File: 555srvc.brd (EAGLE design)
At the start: 34 x 27.9 mm, 11 parts, among them IC2 NE555P

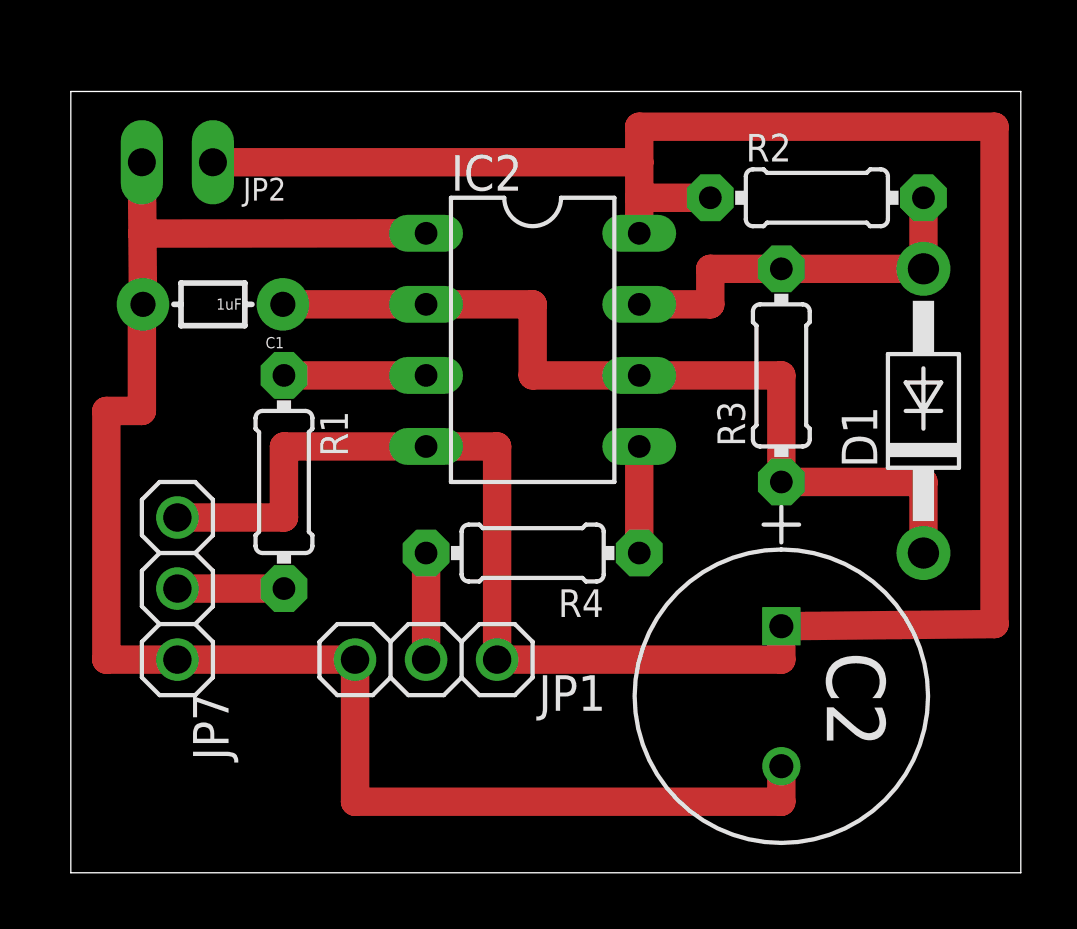
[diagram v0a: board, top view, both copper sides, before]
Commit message: smd is go
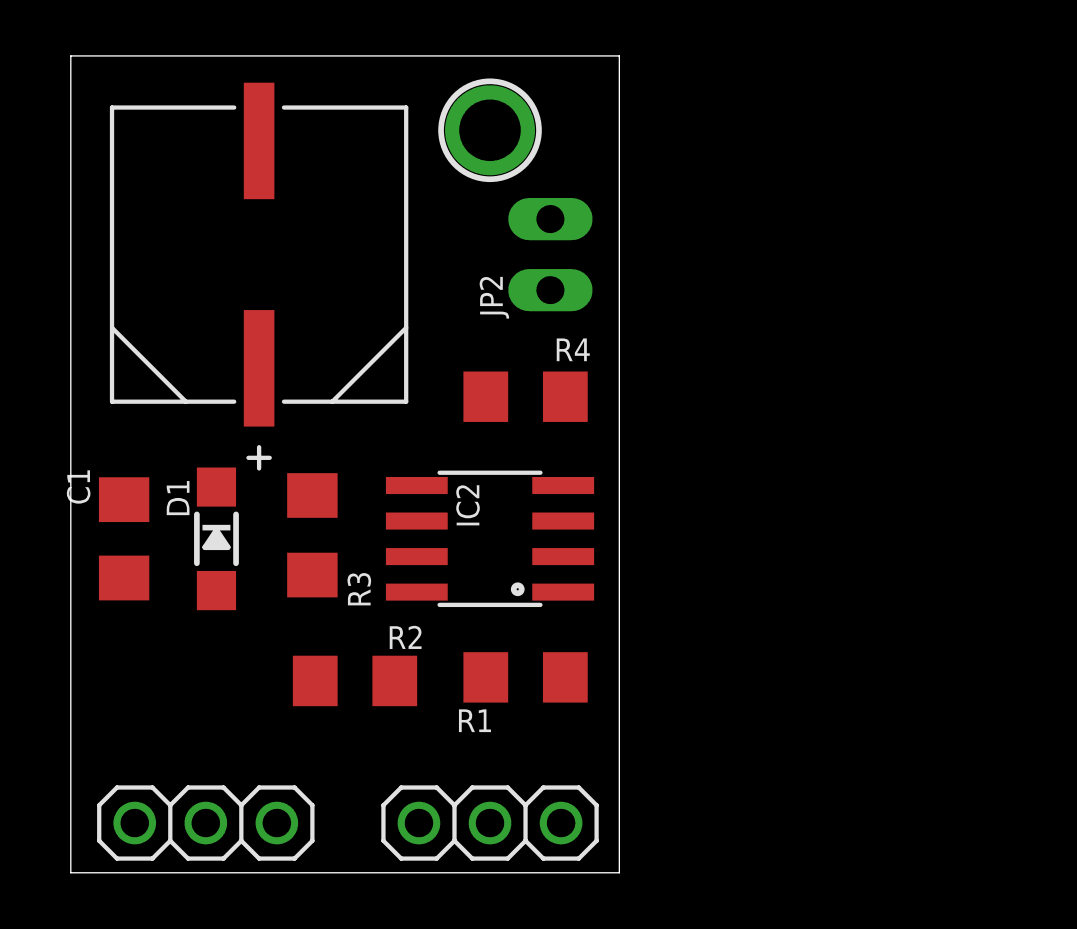
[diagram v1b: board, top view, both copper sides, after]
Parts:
- added U$6: MOUNTINGHOLE2.0, microbuilder:MOUNTINGHOLE_2.0_PLATED
- C1: device SparkFun-Capacitors:AXIAL-5MM -> SparkFun-Capacitors:1206
- C2: device Panasonic-EE4:CAPPR500-1000X3200 -> Panasonic-EEE0_EEE1_EEE2_EEEFC:CAPAE1030X1050N
- D1: value 1N4004 -> (none); device adafruit:DO41-10 -> microbuilder:SOD-123
- IC2: value NE555P -> NE555D; device SparkFun-AnalogIC:DIL-08 -> SparkFun-AnalogIC:SO08
- R1, R2, R3, R4: device adafruit:0204/7 -> adafruit:R1206
- moved C2 26.1 mm to (6.73, 22.1), turned to 90 degrees
- moved D1 25.7 mm to (5.21, 11.9), turned to 270 degrees
- moved R2 23.9 mm to (10.2, 6.86), turned to 180 degrees
- moved R3 17.7 mm to (8.64, 12.1), turned to 270 degrees
- moved JP2 13.7 mm to (17.1, 22.1), turned to 90 degrees
- moved R1 11.1 mm to (16.3, 6.99), turned to 180 degrees
- moved C1 8.96 mm to (1.91, 11.9), turned to 270 degrees
- moved JP7 8.44 mm to (4.83, 1.78), turned to 180 degrees
- moved IC2 7.27 mm to (15.0, 11.9), turned to 90 degrees
- moved JP1 6.27 mm to (15.0, 1.78)
- moved R4 5.59 mm to (16.3, 17.0), turned to 0 degrees
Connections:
- net GND: now also C1.2; no longer C1.P$2
- net N$1: now also C1.1; no longer C1.P$1
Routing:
- net VCC: track 92.6 -> 0.00 mm
- net GND: track 59.7 -> 0.00 mm
- net N$1: track 31.8 -> 0.00 mm
- net N$2: track 14.0 -> 0.00 mm
- net N$5: track 5.08 -> 0.00 mm
- net N$4: track 3.81 -> 0.00 mm
- net SERVO_OUT: track 3.81 -> 0.00 mm
- net INPUT: track 3.81 -> 0.00 mm
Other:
- board size 34 x 27.9 mm -> 19.6 x 29.2 mm
